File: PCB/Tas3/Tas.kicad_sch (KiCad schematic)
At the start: 24 parts, among them J1 Shelly 1, J2 Conn_01x07, J3 USB-C, U1 MD8942, U3 CH340X, U4 ZXGD3009E6, U5 ZXGD3009E6

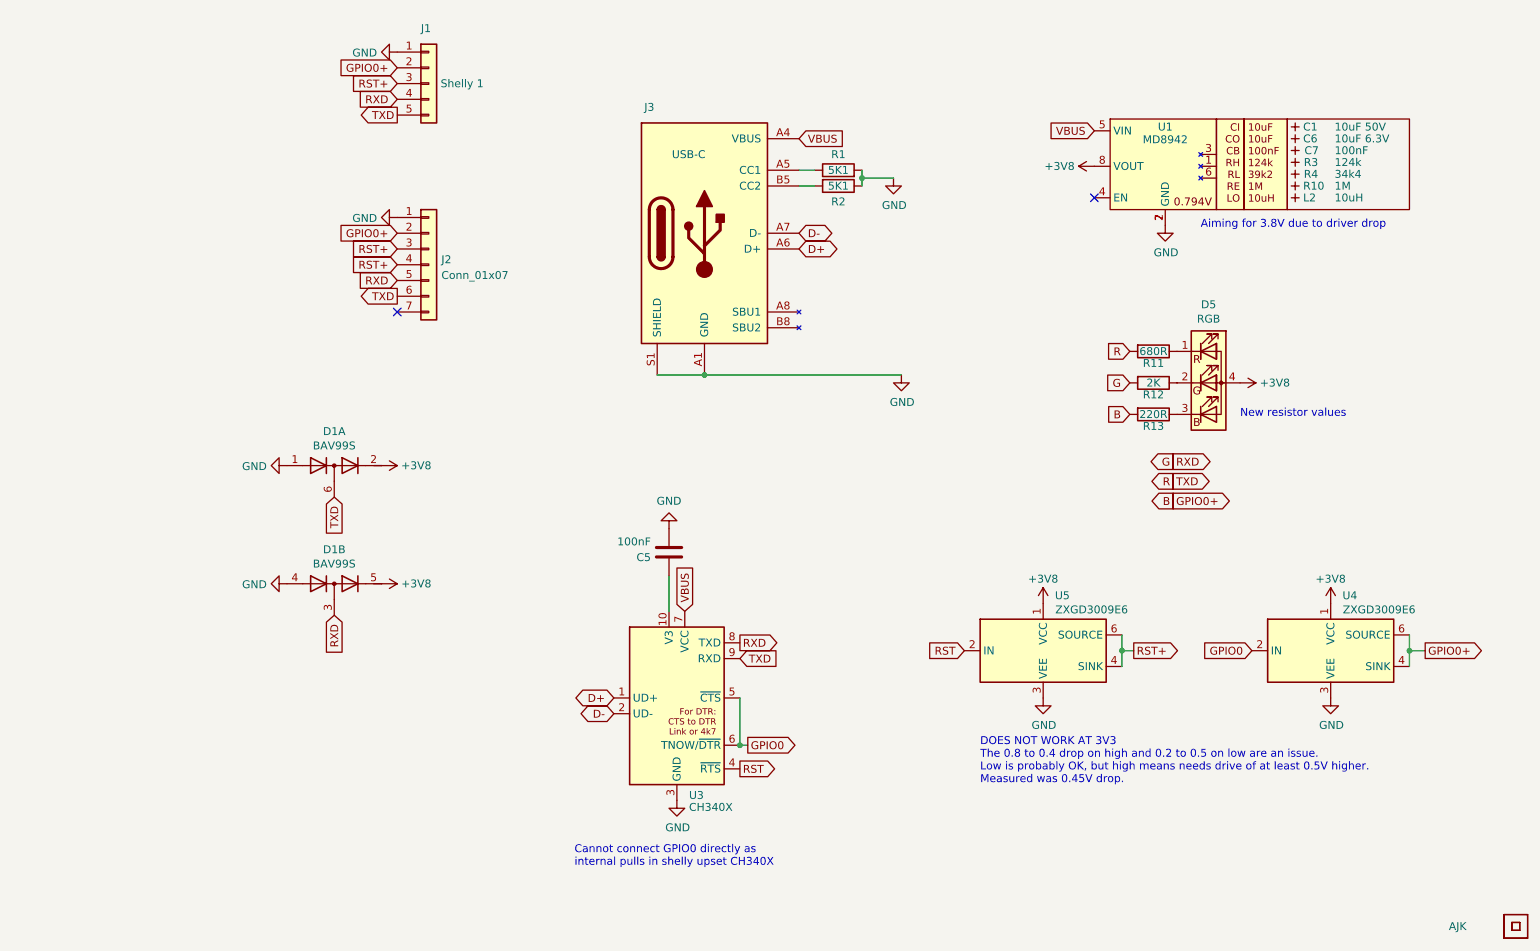
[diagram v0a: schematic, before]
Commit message: Try again, as ordered.
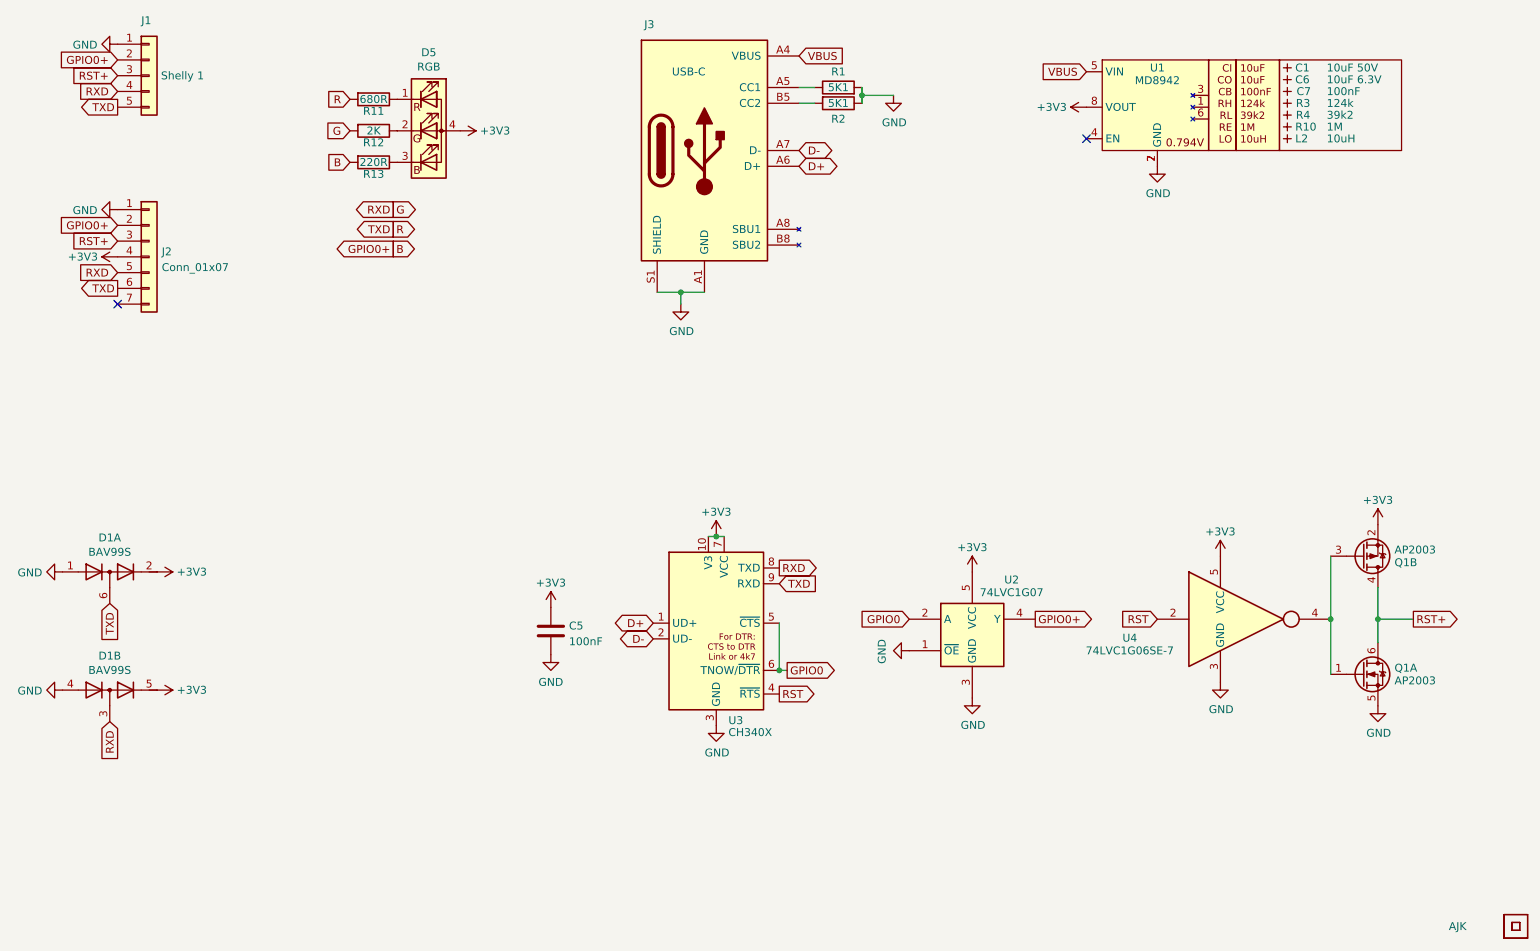
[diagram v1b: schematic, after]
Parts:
- removed U4, U5: ZXGD3009E6, RevK:SOT-23-6, symbol Driver_FET:ZXGD3009E6
- added Q1: AP2003, RevK:SOT-23-6, symbol Transistor_FET:DMC3071LVT
- added U2: 74LVC1G07, RevK:SOT-353_SC-70-5, symbol 74xGxx:NC7SZ125M5X
- added U4: 74LVC1G06SE-7, RevK:SOT-353_SC-70-5, symbol 74xGxx:NC7SVU04P5X
- D1: JLCPCB Rotation Offset -90 -> 0; LCSC Part # C68987 -> C96225
- R4: value 34k4 -> 39k2
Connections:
- net +3V8 is gone; now on net +3V3: D1.2 (K2), D1.5 (K4), D5.4 (A), U1.8 (VOUT)
- net B: now also U2.4 (Y)
- net GND: now also Q1.5 (S), U2.1 (~{OE}), U2.3 (GND), U4.3 (GND)
- net GPIO0: now also U2.2 (A)
- net RST: now also U4.2
- net RST+: now also Q1.4 (D), Q1.6 (D); no longer J2.4 (Pin_4)
- net VBUS: no longer U3.7 (VCC)
- net +3V3: now reaches C5.1, U3.10 (V3)
- net +3V3: now also J2.4 (Pin_4), U3.7 (VCC), Q1.2 (S), U2.5 (VCC), U4.5 (VCC)
- new net: Q1.1 (G), Q1.3 (G), U4.4
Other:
- note removed: "Aiming for 3.8V due to driver drop"
- note removed: "Cannot connect GPIO0 directly as internal pulls in shelly upset CH340X"
- note removed: "DOES NOT WORK AT 3V3 The 0.8 to 0.4 drop on high and 0.2 to 0.5 on low are an issue. Low is probably OK, but high means needs drive of at least 0.5V higher. Measured was 0.45V drop."
- note removed: "New resistor values"
- moved on the sheet: C1, C5, C6, C7, D1A, D1B, D5, J1, J2, J3, L2, R1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
